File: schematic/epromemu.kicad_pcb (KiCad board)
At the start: 2 copper layers, 69.9 x 88.6 mm, 20 parts, among them J3 EPROM Connector, U1 Teensy4.1, U2 74HC245, U3 74HC245, U4 74HC245, U5 74HC245, U6 74HC32

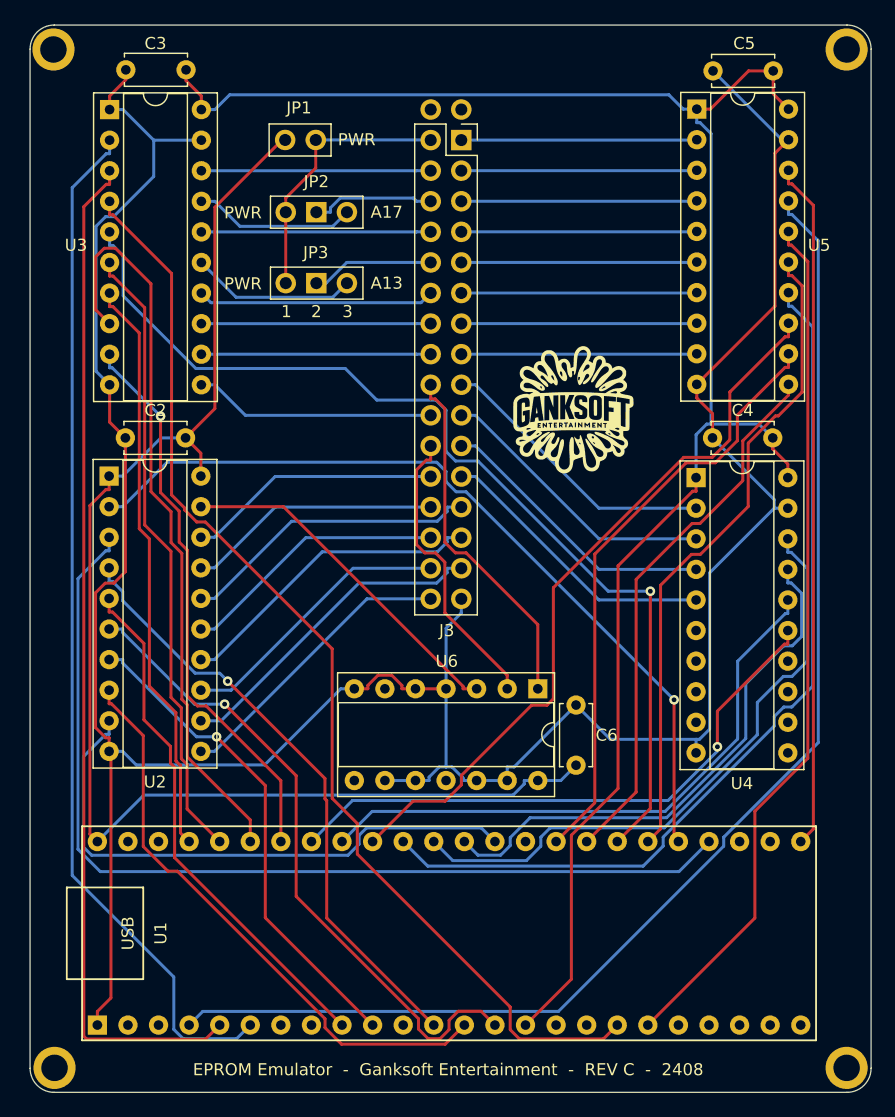
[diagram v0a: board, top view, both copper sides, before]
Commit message: REV D
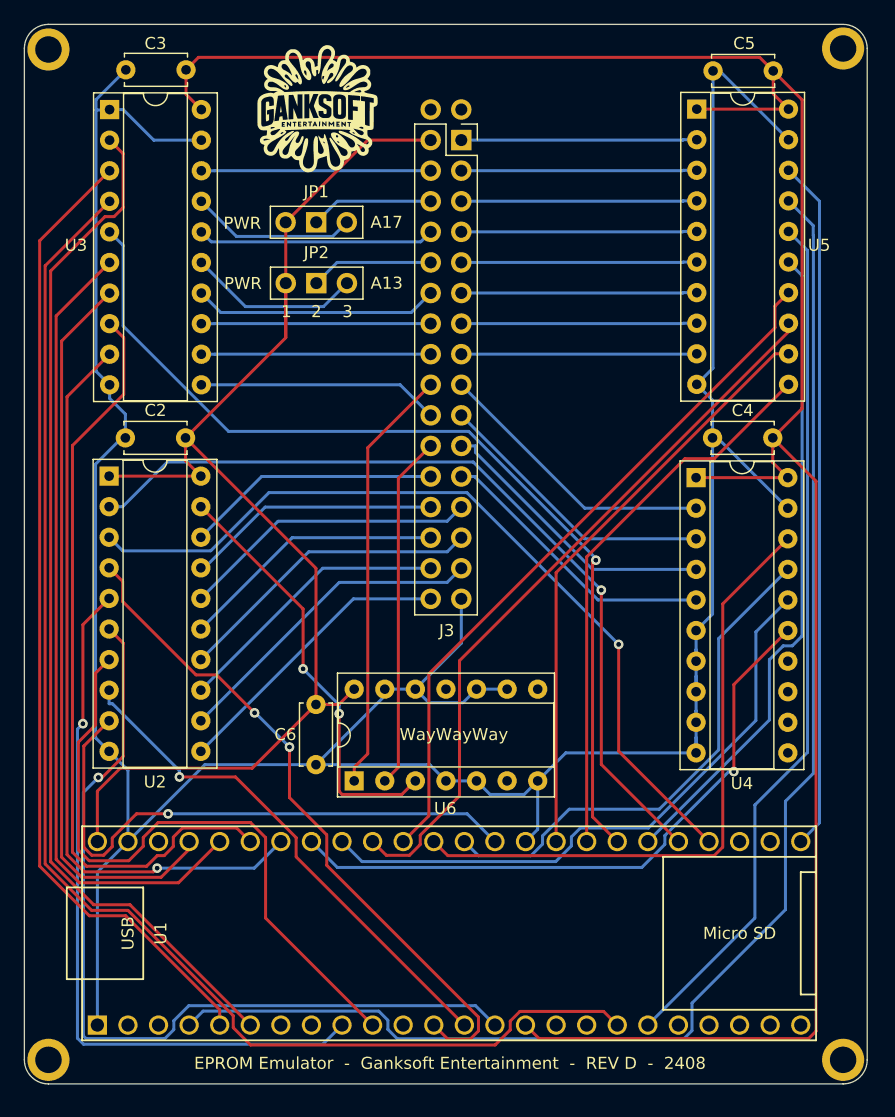
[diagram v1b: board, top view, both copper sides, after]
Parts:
- removed the JP1 at (133.2, 60.6)
- JP1: renamed from JP2; footprint Connector_PinHeader_2.54mm:PinHeader_1x03_P2.54mm_Vertical -> MyFootprints:Jumper_1x03_P2.54mm_Vertical
- JP2: renamed from JP3; footprint Connector_PinHeader_2.54mm:PinHeader_1x03_P2.54mm_Vertical -> MyFootprints:Jumper_1x03_P2.54mm_Vertical
- moved GanksoftLogo 32.8 mm to (133.3, 58.0)
- moved C6 22.2 mm to (133.2, 107.5), turned to -90 degrees
- moved U6 17.1 mm to (136.4, 113.8), turned to 90 degrees
- moved JP1 0.84 mm to (130.7, 67.4)
- moved H4 0.84 mm to (111.0, 137.0)
- moved H3 0.73 mm to (177.0, 137.0)
- moved H1 0.42 mm to (111.0, 53.1)
- moved H2 0.30 mm to (177.0, 53.0)
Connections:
- J3 pad 32: JP1_PWR -> +5V
- JP1 pad 1: JP1_PWR -> +5V
- JP2 pad 1: JP1_PWR -> +5V
- U1 pad 34: unconnected-(U1-GND-Pad34) -> GND
- U1 pad 47: unconnected-(U1-GND-Pad47) -> GND
- U4 pad 6: unconnected-(U4-A4-Pad6) -> GND
- U4 pad 7: unconnected-(U4-A5-Pad7) -> GND
- U4 pad 8: unconnected-(U4-A6-Pad8) -> GND
- U4 pad 9: unconnected-(U4-A7-Pad9) -> GND
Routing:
- net +3V3: track 150.8 -> 184.4 mm
- net JP1_PWR: track 22.5 -> 0.00 mm
- net GND: track 240.8 -> 263.2 mm
- net A14_3V3: track 92.9 -> 113.6 mm
- net D1_3V3: track 54.6 -> 72.4 mm
- net D5_3V3: track 43.6 -> 60.5 mm, vias 0 -> 1
- net A7_3V3: track 75.6 -> 58.8 mm
- net A10_3V3: track 46.9 -> 62.4 mm
- net A8_3V3: track 52.0 -> 67.2 mm
- net D4_3V3: track 41.1 -> 54.3 mm, vias 1 -> 0
- net A9_3V3: track 48.5 -> 61.4 mm
- net D6_3V3: track 81.4 -> 69.5 mm, vias 0 -> 1
- net A16_3V3: track 108.6 -> 117.9 mm
- net D0_3V3: track 50.5 -> 56.7 mm, vias 1 -> 2
- net Net-(U2-CE): track 29.3 -> 35.3 mm, vias 0 -> 2
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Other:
- board size 69.9 x 88.6 mm -> 70 x 88 mm
- board text added: "EPROM Emulator - Ganksoft Entertainment - REV D - 2408"
- board text added: "WayWayWay"
- board text removed: "EPROM Emulator - Ganksoft Entertainment - REV C - 2408"

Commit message: REV E (unproduced)
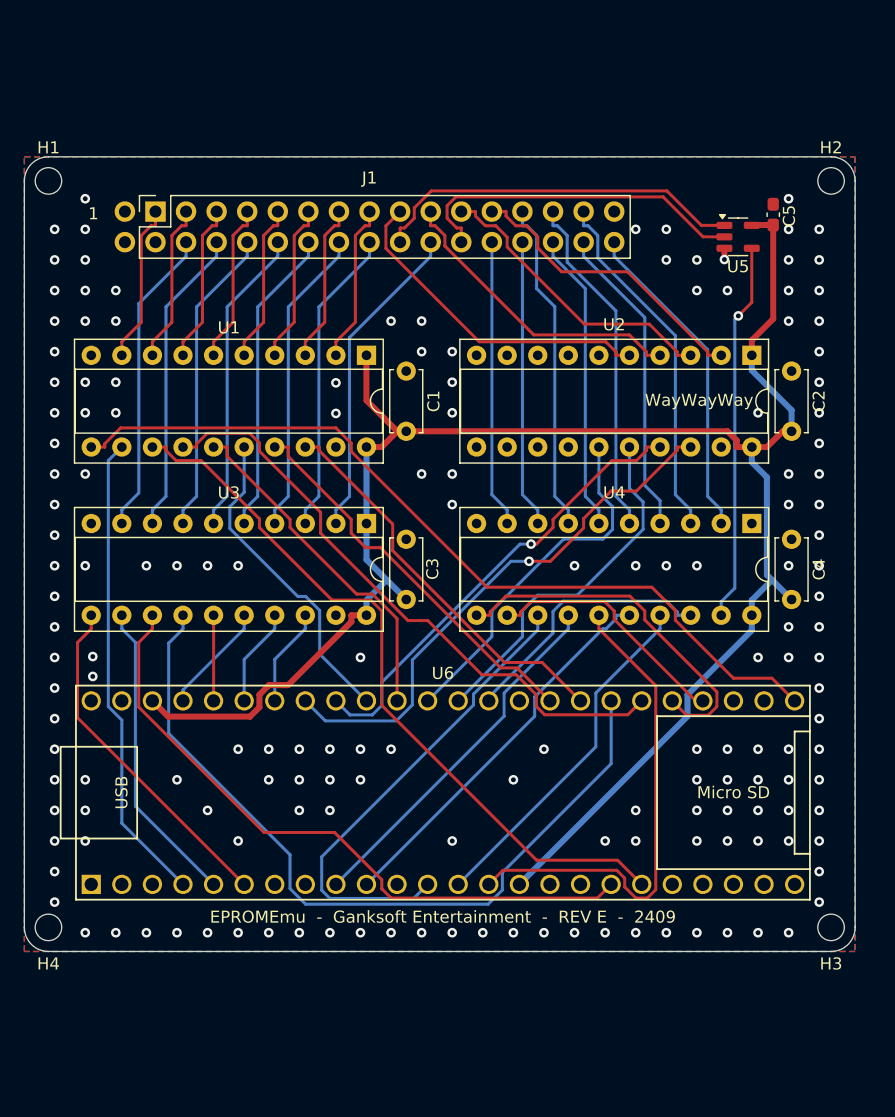
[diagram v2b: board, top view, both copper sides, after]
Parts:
- removed JP1: A17, MyFootprints:Jumper_1x03_P2.54mm_Vertical
- removed JP2: A13, MyFootprints:Jumper_1x03_P2.54mm_Vertical
- C5: renamed from C6; footprint Capacitor_THT:C_Disc_D5.0mm_W2.5mm_P5.00mm -> Capacitor_SMD:C_0603_1608Metric_Pad1.08x0.95mm_HandSolder
- GanksoftLogo: moved to B.Cu
- H1, H2, H3, H4: footprint MountingHole:MountingHole_2.2mm_M2_ISO7380_Pad -> MountingHole:MountingHole_2.2mm_M2_ISO7380
- U1: renamed from U5; value 74HC245 -> SN74LVC245AN
- U2: renamed from U4; value 74HC245 -> SN74LVC245AN
- U3: value 74HC245 -> SN74LVC245AN
- U4: renamed from U2; value 74HC245 -> SN74LVC245AN
- U5: renamed from U6; value 74HC32 -> SN74LVC1G32DBVR; footprint Package_DIP:DIP-14_W7.62mm_Socket -> Package_TO_SOT_SMD:SOT-23-5
- moved GanksoftLogo 56.8 mm to (142.7, 114.0), turned to 180 degrees
- moved C5 55.7 mm to (171.2, 66.8), turned to 90 degrees
- moved U5 55.3 mm to (168.3, 68.6), turned to 0 degrees
- moved U4 53.5 mm to (169.4, 92.5), turned to -90 degrees
- moved C4 52.1 mm to (172.7, 98.8), turned to 90 degrees
- moved C3 47.6 mm to (140.7, 98.8), turned to 90 degrees
- moved C1 42.7 mm to (140.7, 84.8), turned to 90 degrees
- moved U3 40.5 mm to (137.4, 92.5), turned to -90 degrees
- moved U1 34.2 mm to (137.4, 78.5), turned to -90 degrees
- moved J1 24.4 mm to (119.9, 69.1), turned to 90 degrees
- moved U6 11.7 mm to (143.8, 114.8)
- moved U2 11.2 mm to (169.4, 78.5), turned to -90 degrees
- moved H2 11.0 mm to (176.0, 64.0)
- moved H3 11.0 mm to (176.0, 126.0)
- moved H4 11.0 mm to (111.0, 126.0)
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- renumbered C5 to C1, C4 to C2, C2 to C4, J3 to J1, U1 to U6
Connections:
- C4 pad 1: +5V -> +3V3
- C5 pad 1: +5V -> +3V3
- J1 pad 28: Net-(J3-Pin_28) -> A13_5V
- J1 pad 30: Net-(J3-Pin_30) -> A17_5V
- J1 pad 32: +5V -> unconnected-(J1-Pin_32-Pad32)
- U1 pad 11: A4_3V3 -> A19_3V3
- U1 pad 12: A5_3V3 -> A16_3V3
- U1 pad 13: A6_3V3 -> A15_3V3
- U1 pad 14: A7_3V3 -> A12_3V3
- U1 pad 15: A12_3V3 -> A7_3V3
- U1 pad 16: A15_3V3 -> A6_3V3
- U1 pad 17: A16_3V3 -> A5_3V3
- U1 pad 18: A19_3V3 -> A4_3V3
- U1 pad 2: A19_5V -> A4_5V
- U1 pad 3: A16_5V -> A5_5V
- U1 pad 4: A15_5V -> A6_5V
- U1 pad 5: A12_5V -> A7_5V
- U1 pad 6: A7_5V -> A12_5V
- U1 pad 7: A6_5V -> A15_5V
- U1 pad 8: A5_5V -> A16_5V
- U1 pad 9: A4_5V -> A19_5V
- U2 pad 15: A0_3V3 -> A3_3V3
- U2 pad 16: A1_3V3 -> A2_3V3
- U2 pad 17: A2_3V3 -> A1_3V3
- U2 pad 18: A3_3V3 -> A0_3V3
- U2 pad 2: A3_5V -> A0_5V
- U2 pad 3: A2_5V -> A1_5V
- U2 pad 4: A1_5V -> A2_5V
- U2 pad 5: A0_5V -> A3_5V
- U3 pad 1: GND -> +3V3
- U3 pad 11: A10_5V -> A18_3V3
- U3 pad 12: A11_5V -> A17_3V3
- U3 pad 13: A9_5V -> A14_3V3
- U3 pad 14: A8_5V -> A13_3V3
- U3 pad 15: A13_5V -> A8_3V3
- U3 pad 16: A14_5V -> A9_3V3
- U3 pad 17: A17_5V -> A11_3V3
- U3 pad 18: A18_5V -> A10_3V3
- U3 pad 2: A18_3V3 -> A10_5V
- U3 pad 3: A17_3V3 -> A11_5V
- U3 pad 4: A14_3V3 -> A9_5V
- U3 pad 5: A13_3V3 -> A8_5V
- U3 pad 6: A8_3V3 -> A13_5V
- U3 pad 7: A9_3V3 -> A14_5V
- U3 pad 8: A11_3V3 -> A17_5V
- U3 pad 9: A10_3V3 -> A18_5V
- U4 pad 1: +5V -> GND
- U4 pad 11: D3_5V -> D7_3V3
- U4 pad 12: D2_5V -> D6_3V3
- U4 pad 13: D4_5V -> D0_3V3
- U4 pad 14: D1_5V -> D5_3V3
- U4 pad 15: D5_5V -> D1_3V3
- U4 pad 16: D0_5V -> D4_3V3
- U4 pad 17: D6_5V -> D2_3V3
- U4 pad 18: D7_5V -> D3_3V3
- U4 pad 19: Net-(U2-CE) -> OE_CE
- U4 pad 2: D7_3V3 -> D3_5V
- U4 pad 20: +5V -> +3V3
- U4 pad 3: D6_3V3 -> D2_5V
- U4 pad 4: D0_3V3 -> D4_5V
- U4 pad 5: D5_3V3 -> D1_5V
- U4 pad 6: D1_3V3 -> D5_5V
- U4 pad 7: D4_3V3 -> D0_5V
- U4 pad 8: D2_3V3 -> D6_5V
- U4 pad 9: D3_3V3 -> D7_5V
- U5 pad 3: Net-(U2-CE) -> GND
- U5 pad 4: GND -> OE_CE
- U5 pad 5: GND -> +3V3
- U6 pad 46: unconnected-(U1-3V3-Pad46) -> +3V3
- U6 pad 48: +5V -> unconnected-(U6-VIN-Pad48)
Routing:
- net GND: track 263.2 -> 0.93 mm, vias 0 -> 164
- net +5V: track 107.7 -> 0.00 mm
- net A16_3V3: track 117.9 -> 39.4 mm
- net A8_3V3: track 67.2 -> 7.11 mm
- net A14_3V3: track 113.6 -> 54.8 mm
- net A18_3V3: track 85.5 -> 28.6 mm
- net A17_3V3: track 81.3 -> 25.5 mm
- net A11_3V3: track 63.6 -> 8.16 mm
- net A10_3V3: track 62.4 -> 8.16 mm, vias 1 -> 0
- net A9_3V3: track 61.4 -> 9.22 mm
- net D6_3V3: track 69.5 -> 20.1 mm, vias 1 -> 0
- net D7_3V3: track 70.4 -> 30.2 mm, vias 1 -> 0
- net Net-(U2-CE): track 35.3 -> 0.00 mm, vias 2 -> 0
- net A6_3V3: track 60.8 -> 26.7 mm
- net D1_3V3: track 72.4 -> 40.8 mm, vias 1 -> 0
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- added copper zone on B.Cu, net GND
- added copper zone on F.Cu, net GND
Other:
- board size 70 x 88 mm -> 69 x 66 mm
- board text added: "C3"
- board text added: "EPROMEmu - Ganksoft Entertainment - REV E - 2409"
- board text removed: "2"
- board text removed: "3"
- board text removed: "EPROM Emulator - Ganksoft Entertainment - REV D - 2408"
- board text removed: "PWR"

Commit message: REV F
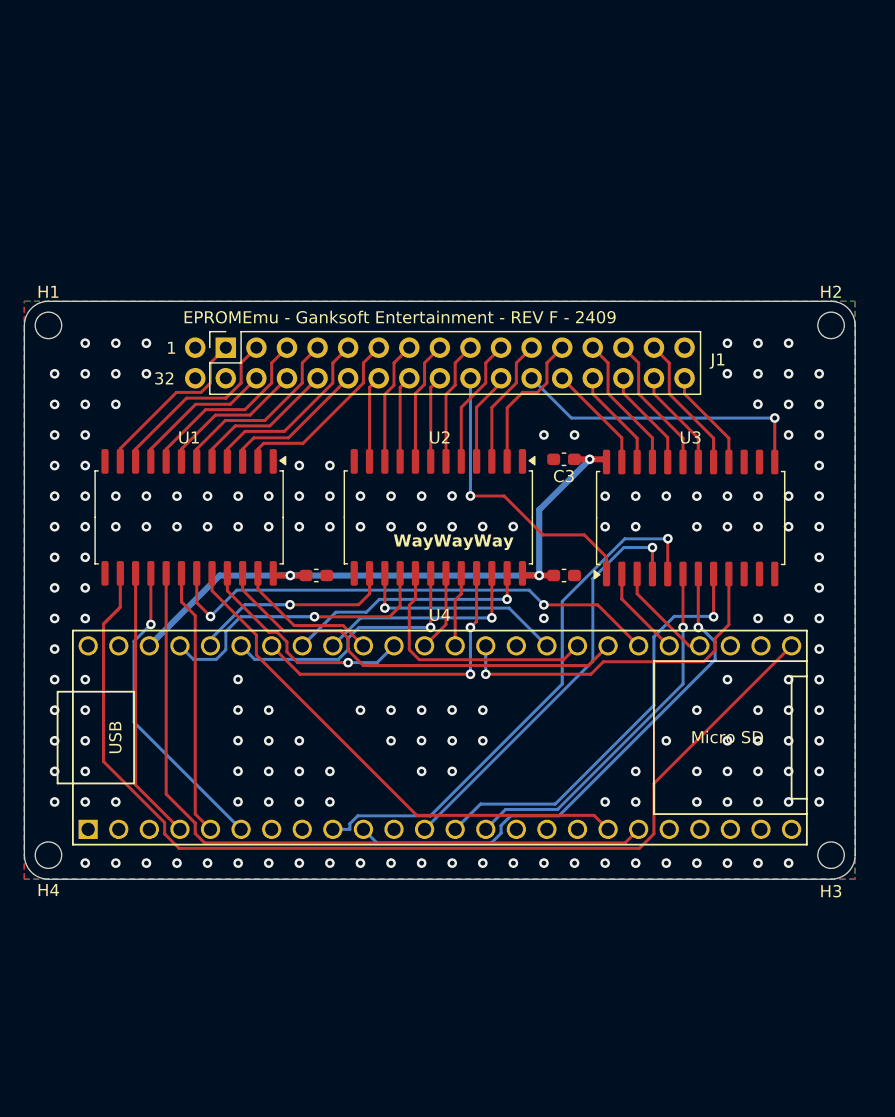
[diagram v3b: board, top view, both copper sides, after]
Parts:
- removed the C1 at (140.7, 84.8)
- removed C5: 0.1uf, Capacitor_SMD:C_0603_1608Metric_Pad1.08x0.95mm_HandSolder
- removed the U4 at (169.4, 92.5)
- removed U5: SN74LVC1G32DBVR, Package_TO_SOT_SMD:SOT-23-5
- C1: renamed from C3; footprint Capacitor_THT:C_Disc_D5.0mm_W2.5mm_P5.00mm -> Capacitor_SMD:C_0603_1608Metric_Pad1.08x0.95mm_HandSolder
- C2: footprint Capacitor_THT:C_Disc_D5.0mm_W2.5mm_P5.00mm -> Capacitor_SMD:C_0603_1608Metric_Pad1.08x0.95mm_HandSolder
- C3: renamed from C4; footprint Capacitor_THT:C_Disc_D5.0mm_W2.5mm_P5.00mm -> Capacitor_SMD:C_0603_1608Metric_Pad1.08x0.95mm_HandSolder
- U1, U2, U3: value SN74LVC245AN -> SN74LVC827APWR; footprint Package_DIP:DIP-20_W7.62mm_Socket -> Package_SO:SOIC-24W_7.5x15.4mm_P1.27mm
- moved U2 29.3 mm to (143.4, 91.9)
- moved U3 26.9 mm to (164.3, 92.0), turned to 90 degrees
- moved C2 22.4 mm to (153.8, 96.8), turned to 0 degrees
- moved C3 22.2 mm to (153.8, 87.1), turned to 180 degrees
- moved U1 20.0 mm to (122.7, 91.9)
- moved J1 12.7 mm to (125.7, 80.4)
- moved H1 12.0 mm to (111.0, 76.0)
- moved H2 12.0 mm to (176.0, 76.0)
- moved C1 7.73 mm to (133.2, 96.8), turned to 0 degrees
- moved H3 6.00 mm to (176.0, 120.0)
- moved H4 6.00 mm to (111.0, 120.0)
- moved U4 4.58 mm to (143.5, 110.2)
- moved GanksoftLogo 3.81 mm to (142.9, 110.2)
- renumbered U6 to U4
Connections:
- U1 pad 1: +3V3 -> GND
- U1 pad 10: GND -> A16_5V
- U1 pad 11: A19_3V3 -> A19_5V
- U1 pad 12: A16_3V3 -> GND
- U1 pad 13: A15_3V3 -> GND
- U1 pad 14: A12_3V3 -> A19_3V3
- U1 pad 15: A7_3V3 -> A16_3V3
- U1 pad 16: A6_3V3 -> A18_3V3
- U1 pad 17: A5_3V3 -> A15_3V3
- U1 pad 18: A4_3V3 -> A17_3V3
- U1 pad 19: GND -> A12_3V3
- U1 pad 2: A4_5V -> A6_5V
- U1 pad 20: +3V3 -> A14_3V3
- U1 pad 3: A5_5V -> A13_5V
- U1 pad 4: A6_5V -> A7_5V
- U1 pad 5: A7_5V -> A14_5V
- U1 pad 7: A15_5V -> A17_5V
- U1 pad 8: A16_5V -> A15_5V
- U1 pad 9: A19_5V -> A18_5V
- U2 pad 1: +3V3 -> GND
- U2 pad 10: GND -> A5_5V
- U2 pad 11: unconnected-(U2-B7-Pad11) -> A8_5V
- U2 pad 12: unconnected-(U2-B6-Pad12) -> GND
- U2 pad 13: unconnected-(U2-B5-Pad13) -> GND
- U2 pad 14: unconnected-(U2-B4-Pad14) -> A8_3V3
- U2 pad 15: A3_3V3 -> A5_3V3
- U2 pad 16: A2_3V3 -> A9_3V3
- U2 pad 17: A1_3V3 -> A4_3V3
- U2 pad 18: A0_3V3 -> A11_3V3
- U2 pad 19: GND -> A3_3V3
- U2 pad 20: +3V3 -> A2_3V3
- U2 pad 4: A2_5V -> A10_5V
- U2 pad 5: A3_5V -> A2_5V
- U2 pad 6: GND -> A3_5V
- U2 pad 7: GND -> A11_5V
- U2 pad 8: GND -> A4_5V
- U2 pad 9: GND -> A9_5V
- U3 pad 1: +3V3 -> OE_5V
- U3 pad 11: A18_3V3 -> GND
- U3 pad 12: A17_3V3 -> GND
- U3 pad 13: A14_3V3 -> CE_5V
- U3 pad 14: A13_3V3 -> unconnected-(U3-Y1O-Pad14)
- U3 pad 15: A8_3V3 -> unconnected-(U3-Y9-Pad15)
- U3 pad 16: A9_3V3 -> D3_5V
- U3 pad 17: A11_3V3 -> D2_5V
- U3 pad 18: A10_3V3 -> D4_5V
- U3 pad 19: GND -> D1_5V
- U3 pad 2: A10_5V -> D7_3V3
- U3 pad 20: +3V3 -> D5_5V
- U3 pad 3: A11_5V -> D6_3V3
- U3 pad 4: A9_5V -> D0_3V3
- U3 pad 5: A8_5V -> D5_3V3
- U3 pad 6: A13_5V -> D1_3V3
- U3 pad 7: A14_5V -> D4_3V3
- U3 pad 8: A17_5V -> D2_3V3
- U3 pad 9: A18_5V -> D3_3V3
- U4 pad 15: +3V3 -> unconnected-(U4-3V3-Pad15)
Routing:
- net +3V3: track 154.0 -> 54.4 mm, vias 0 -> 3
- net OE_CE: track 31.5 -> 0.00 mm, vias 1 -> 0
- net A13_3V3: track 65.5 -> 35.6 mm
- net A0_3V3: track 44.9 -> 20.8 mm
- net A2_3V3: track 29.8 -> 6.23 mm
- net A3_3V3: track 29.8 -> 6.75 mm
- net D7_3V3: track 30.2 -> 7.58 mm
- net A1_3V3: track 38.3 -> 17.9 mm
- net A10_5V: track 26.6 -> 7.75 mm
- net A19_3V3: track 69.5 -> 88.2 mm
- net D3_5V: track 27.1 -> 8.48 mm
- net A11_5V: track 25.6 -> 7.22 mm
- net A8_5V: track 25.6 -> 7.22 mm
- net A9_5V: track 25.6 -> 7.22 mm
- net D2_5V: track 29.8 -> 11.5 mm
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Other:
- board size 69 x 66 mm -> 69 x 48 mm
- board text added: "32"
- board text added: "EPROMEmu - Ganksoft Entertainment - REV F - 2409"
- board text removed: "C3"
- board text removed: "EPROMEmu - Ganksoft Entertainment - REV E - 2409"
